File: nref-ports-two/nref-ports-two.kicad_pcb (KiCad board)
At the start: 4 copper layers, 87.5 x 40.2 mm, 117 parts, among them J1 USB_C_Receptacle, J2 USB_C_Receptacle, J3 USB3_A, J4 HD0919MSMTTR, J5 Conn_01x20, J6 Conn_01x12_Pin, J7 Conn_01x04, U1 TUSB8041, U10 TPD4E02B04DQA, U11 TPD12S521, U12 LM2830XQMFE/NOPB, U13 LM2830XQMFE/NOPB, U2 HD3SS3220IRNHT, U3 TPD4E02B04DQA, U4 TPD4E02B04DQA, U5 TPD4E02B04DQA, U6 TPD4E02B04DQA, U7 TPD4E02B04DQA, U8 TPD4E02B04DQA, U9 TPD4E02B04DQA, Y1 24MHz

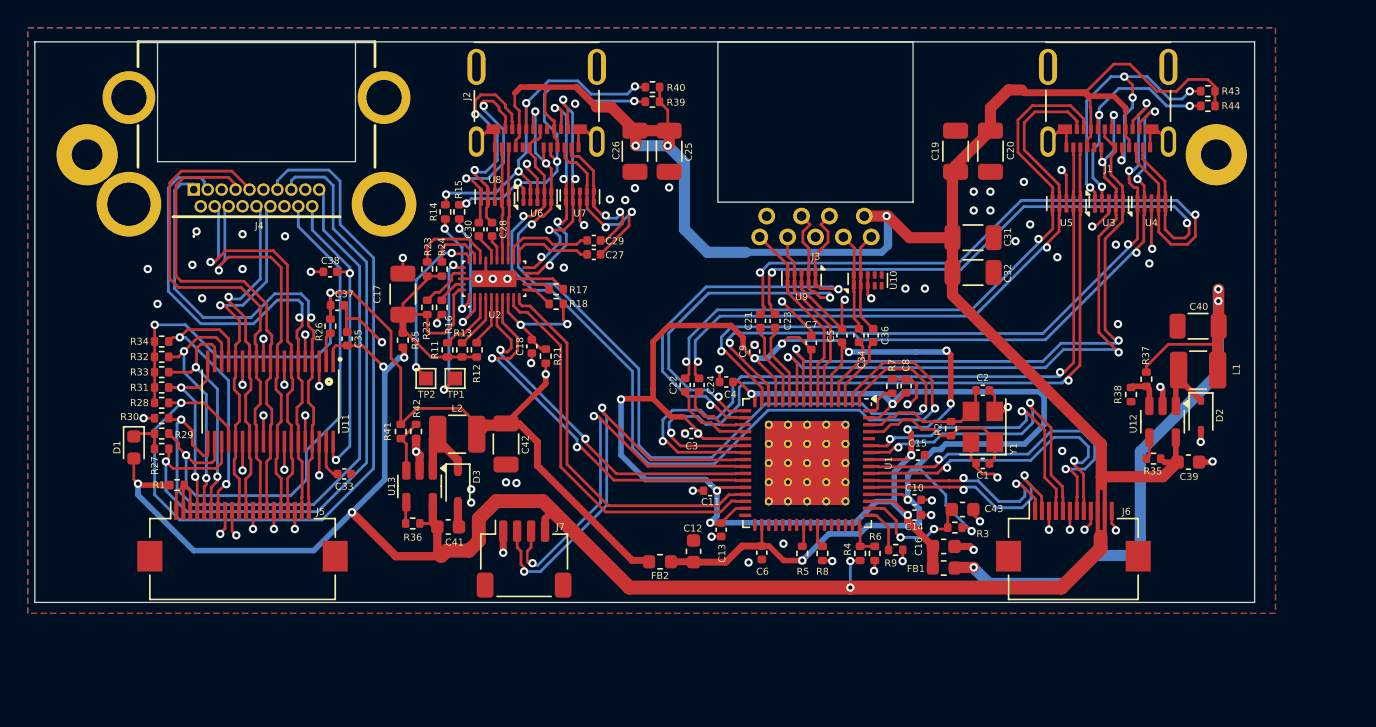
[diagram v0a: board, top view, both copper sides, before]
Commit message: WIP ports-two redesign
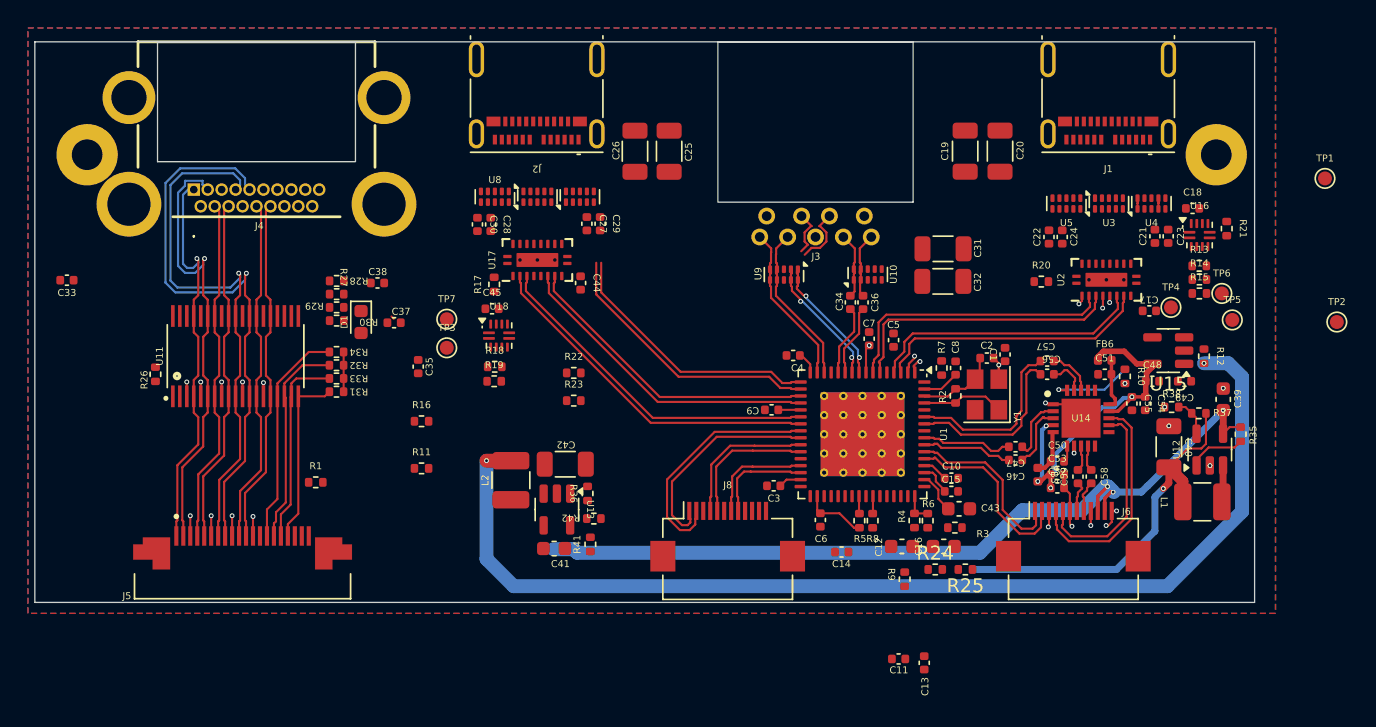
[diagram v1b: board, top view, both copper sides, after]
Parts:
- removed D2, D3: PMEG1020EA,115, Diode_SMD:D_SOD-323
- removed FB1, FB2: 220@100MHz 1.4A, Inductor_SMD:L_0603_1608Metric
- removed J7: Conn_01x04, Connector_JST:JST_SH_SM04B-SRSS-TB_1x04-1MP_P1.00mm_Horizontal
- removed R39, R40, R43, R44: 22k, Resistor_SMD:R_0402_1005Metric
- added C44: 0.1uF, Capacitor_SMD:C_0402_1005Metric, F.Cu at (139.2, 97.3)
- added C45: 0.1uF, Capacitor_SMD:C_0402_1005Metric, F.Cu at (132.8, 99.2)
- added C46: 0.1uF, Capacitor_SMD:C_0402_1005Metric, F.Cu at (170.3, 110.0)
- added C47: 0.1uF, Capacitor_SMD:C_0402_1005Metric, F.Cu at (170.3, 109.0)
- added C48: 1uF, Capacitor_SMD:C_0402_1005Metric, F.Cu at (180.2, 104.3)
- added C49: 1uF, Capacitor_SMD:C_0402_1005Metric, F.Cu at (182.5, 104.3)
- added C50: 4.7uF, Capacitor_SMD:C_0402_1005Metric, F.Cu at (173.3, 110.1)
- added C51: 4.7uF, Capacitor_SMD:C_0402_1005Metric, F.Cu at (176.8, 103.8)
- added C52: 0.1uF, Capacitor_SMD:C_0402_1005Metric, F.Cu at (173.3, 112.0)
- added C53: 1uF, Capacitor_SMD:C_0402_1005Metric, F.Cu at (173.3, 111.0)
- added C54: 1uF, Capacitor_SMD:C_0402_1005Metric, F.Cu at (179.7, 106.0)
- added C55: 0.1uF, Capacitor_SMD:C_0402_1005Metric, F.Cu at (178.7, 106.0)
- added C56: 0.1uF, Capacitor_SMD:C_0402_1005Metric, F.Cu at (172.6, 103.8)
- added C57: 0.1uF, Capacitor_SMD:C_0402_1005Metric, F.Cu at (172.6, 102.9)
- added C58: 0.1uF, Capacitor_SMD:C_0402_1005Metric, F.Cu at (175.8, 111.2)
- added C59: 0.1uF, Capacitor_SMD:C_0402_1005Metric, F.Cu at (174.8, 111.2)
- added FB5: 100@100MHz 3A, Inductor_SMD:L_0402_1005Metric, F.Cu at (171.9, 111.0)
- added FB6: 100@100MHz 3A, Inductor_SMD:L_0402_1005Metric, F.Cu at (176.8, 102.8)
- added J8: Conn_01x12_Pin, Connector_FFC-FPC:Hirose_FH12-12S-0.5SH_1x12-1MP_P0.50mm_Horizontal, F.Cu at (149.7, 115.5)
- added R10: 0, Resistor_SMD:R_0402_1005Metric, F.Cu at (178.2, 104.0)
- added R19: 900k, Resistor_SMD:R_0402_1005Metric, F.Cu at (132.9, 104.3)
- added R20: 0, Resistor_SMD:R_0402_1005Metric, F.Cu at (172.2, 97.2)
- added TP3: TestPoint, TestPoint:TestPoint_Pad_D1.0mm, F.Cu at (129.6, 102.0)
- added TP4: TestPoint, TestPoint:TestPoint_Pad_D1.0mm, F.Cu at (181.5, 99.0)
- added TP5: TestPoint, TestPoint:TestPoint_Pad_D1.0mm, F.Cu at (185.9, 100.0)
- added TP6: TestPoint, TestPoint:TestPoint_Pad_D1.0mm, F.Cu at (185.2, 98.0)
- added TP7: TestPoint, TestPoint:TestPoint_Pad_D1.0mm, F.Cu at (129.6, 99.9)
- added U14: EQCO5X31C0-I_6NX, footprints:QFN50P400X400X100-21N-D, F.Cu at (175.1, 107.0)
- added U15: LP5907MFX-1.2, Package_TO_SOT_SMD:SOT-23-5, F.Cu at (181.3, 102.2)
- added U16: TUSB321, Package_DFN_QFN:Texas_X2QFN-12_1.6x1.6mm_P0.4mm, F.Cu at (183.6, 93.9)
- added U17: TMUXHS4212, footprints:Texas-VQFN20_2.5x4.5mm_RKS, F.Cu at (136.1, 95.7)
- added U18: TUSB321, Package_DFN_QFN:Texas_X2QFN-12_1.6x1.6mm_P0.4mm, F.Cu at (133.3, 101.1)
- C17: value 47uF -> 0.1uF; footprint Capacitor_SMD:C_1206_3216Metric -> Capacitor_SMD:C_0402_1005Metric
- J1, J2: footprint footprints:MOLEX_105450-0101 -> Connector_USB:USB_C_Receptacle_Molex_105450-0101
- J5: footprint Connector_FFC-FPC:Hirose_FH12-20S-0.5SH_1x20-1MP_P0.50mm_Horizontal -> footprints:AMPHENOL_SFV20R-2STE1HLF
- R11: value 10k -> 0
- R12: value 900k -> 10k
- R13, R22: value 200k -> 10k
- R14: value 0 -> 4.7k
- R15: value 0 -> 900k
- R18, R24: value 200k -> 0
- R23: value 200k -> 4.7k
- R31, R35, R36: value 100k -> 10k
- TP1, TP2: footprint TestPoint:TestPoint_Pad_1.0x1.0mm -> TestPoint:TestPoint_Pad_D1.0mm
- U12, U13: value LM2830XQMFE/NOPB -> TLV62569DBV
- U2: value HD3SS3220IRNHT -> TMUXHS4212; footprint footprints:QFN40P450X250X80-31N120X320 -> footprints:Texas-VQFN20_2.5x4.5mm_RKS
- moved TP2 65.5 mm to (193.4, 100.1)
- moved TP1 64.0 mm to (192.6, 89.8)
- moved R14 54.3 mm to (183.5, 97.0), turned to 0 degrees
- moved C17 53.6 mm to (179.9, 99.3), turned to 0 degrees
- moved R15 53.4 mm to (183.5, 98.0), turned to 0 degrees
- moved R13 53.2 mm to (183.5, 96.1), turned to 0 degrees
- moved R12 52.2 mm to (183.9, 102.5), turned to -90 degrees
- moved R21 49.7 mm to (185.5, 93.4)
- moved C18 48.4 mm to (183.1, 92.0), turned to 0 degrees
- moved U2 43.9 mm to (176.9, 97.1)
- moved R25 43.6 mm to (166.8, 117.8), turned to 180 degrees
- moved R24 41.4 mm to (164.6, 117.8), turned to 0 degrees
- moved C21 28.9 mm to (180.3, 94.0)
- moved C23 28.8 mm to (181.3, 94.0)
- moved C22 28.2 mm to (172.8, 94.0)
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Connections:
- net /USB3_1_SSTXCN renamed /USBH3_TXCN
- net /USB3_1_SSTXCP renamed /USBH3_TXCP
- net /USBH_1A_AC_TXN renamed /USBC2A_TXCN
- net /USBH_1A_AC_TXP renamed /USBC2A_TXCP
- net /USBH_1B_AC_TXN renamed /USBC2B_TXCN
- net /USBH_1B_AC_TXP renamed /USBC2B_TXCP
- net /USBH_2A_AC_TXN renamed /USBC1A_TXCN
- net /USBH_2A_AC_TXP renamed /USBC1A_TXCP
- net /USBH_2B_AC_TXN renamed /USBC1B_TXCN
- net /USBH_2B_AC_TXP renamed /USBC1B_TXCP
- net CC1 renamed USBC1_CC1
- net CC2 renamed USBC1_CC2
- C17 pad 1: MUX_5V -> /MUX_3V3
- C18 pad 1: MUX_3V3 -> +5V
- C21 pad 2: USBH_2A_TXN -> USBC1A_TXN
- C22 pad 2: USBH_2B_TXN -> USBC1B_TXN
- C23 pad 2: USBH_2A_TXP -> USBC1A_TXP
- C24 pad 2: USBH_2B_TXP -> USBC1B_TXP
- C27 pad 2: USBH_MUXA_TXN -> USBC2A_TXN
- C28 pad 2: USBH_MUXB_TXN -> USBC2B_TXN
- C29 pad 2: USBH_MUXA_TXP -> USBC2A_TXP
- C30 pad 2: USBH_MUXB_TXP -> USBC2B_TXP
- C34 pad 1: USBH_1A_TXN -> USBH3_TXN
- C36 pad 1: USBH_1A_TXP -> USBH3_TXP
- J1 pad A10: USBH_2B_RXN -> USBC1B_RXN
- J1 pad A11: USBH_2B_RXP -> USBC1B_RXP
- J1 pad A6: USBH_2_DP -> USBC1_DP
- J1 pad A7: USBH_2_DN -> USBC1_DN
- J1 pad B10: USBH_2A_RXN -> USBC1A_RXN
- J1 pad B11: USBH_2A_RXP -> USBC1A_RXP
- J1 pad B6: USBH_2_DP -> USBC1_DP
- J1 pad B7: USBH_2_DN -> USBC1_DN
- J2 pad A10: USBH_MUXB_RXN -> USBC2B_RXN
- J2 pad A11: USBH_MUXB_RXP -> USBC2B_RXP
- J2 pad A5: MUXCC1 -> USBC2_CC1
- J2 pad A6: USBH_1_DP -> USBC2_DP
- J2 pad A7: USBH_1_DN -> USBC2_DN
- J2 pad B10: USBH_MUXA_RXN -> USBC2A_RXN
- J2 pad B11: USBH_MUXA_RXP -> USBC2A_RXP
- J2 pad B5: MUXCC2 -> USBC2_CC2
- J2 pad B6: USBH_1_DP -> USBC2_DP
- J2 pad B7: USBH_1_DN -> USBC2_DN
- J3 pad 5: USBH_1A_RXN -> USBH3_RXN
- J3 pad 6: USBH_1A_RXP -> USBH3_RXP
- J5 pad 1: Net-(J5-Pin_1) -> HDMI_TX2P
- J5 pad 10: HDMI_CLKN -> HDMI_CLKP
- J5 pad 11: HDMI_CLKP -> HDMI_CLKN
- J5 pad 13: HDMI_TX0N -> GND
- J5 pad 14: HDMI_TX0P -> HDMI_CEC
- J5 pad 15: GND -> HDMI_SCL
- J5 pad 16: HDMI_TX1N -> HDMI_SDA
- J5 pad 17: HDMI_TX1P -> HDMI_HPD
- J5 pad 18: GND -> Net-(J5-Pin_18)
- J5 pad 19: HDMI_TX2N -> Net-(J5-Pin_18)
- J5 pad 2: Net-(J5-Pin_1) -> HDMI_TX2N
- J5 pad 20: HDMI_TX2P -> Net-(J5-Pin_18)
- J5 pad 3: Net-(J5-Pin_1) -> GND
- J5 pad 4: HDMI_HPD -> HDMI_TX1P
- J5 pad 5: HDMI_SCL -> HDMI_TX1N
- J5 pad 6: HDMI_SDA -> GND
- J5 pad 7: HDMI_CEC -> HDMI_TX0P
- J5 pad 8: GND -> HDMI_TX0N
- L1 pad 1: Net-(D2-K) -> Net-(U12-SW)
- L2 pad 1: Net-(D3-K) -> Net-(U13-SW)
- R1 pad 1: Net-(J5-Pin_1) -> Net-(J5-Pin_18)
- R11 pad 1: MUX_5V -> /MUX_3V3
- R11 pad 2: Net-(U2-CURRENT_MODE) -> +3V3
- R12 pad 1: MUX_5V -> Net-(U15-EN)
- R12 pad 2: Net-(U2-VBUS_DET) -> +3V3
- R13 pad 1: MUX_5V -> +5V
- R13 pad 2: Net-(U2-PORT) -> Net-(U16-CURRENT_MODE)
- R14 pad 1: MUXCC2 -> +5V
- R14 pad 2: Net-(U2-CC2) -> Net-(U16-PORT)
- R15 pad 1: MUXCC1 -> +5V
- R15 pad 2: Net-(U2-CC1) -> Net-(U16-VBUS_DET)
- R16 pad 1: GND -> /MUX_3V3
- R16 pad 2: Net-(U2-~{ENN_CC}) -> +3V3
- R17 pad 1: GND -> ~{USB_MUX_OE}
- R17 pad 2: Net-(U2-~{ENN_MUX}) -> Net-(U17-~{OE})
- R18 pad 1: Net-(U2-DIR) -> USBC2_MUX_DIR
- R18 pad 2: MUX_3V3 -> Net-(U17-SEL)
- R21 pad 1: MUX_3V3 -> USBC1_MUX_DIR
- R21 pad 2: +3V3 -> Net-(U2-SEL)
- R22 pad 1: Net-(U2-ID) -> +5V
- R22 pad 2: MUX_5V -> Net-(U18-CURRENT_MODE)
- R23 pad 1: Net-(U2-~{INT_N}/OUT3) -> +5V
- R23 pad 2: MUX_5V -> Net-(U18-PORT)
- R24 pad 1: Net-(U2-VCONN_FAULT_N) -> +3V3
- R24 pad 2: MUX_5V -> USBH_3V3
- R25 pad 1: MUX_5V -> +1V1
- R25 pad 2: +5V -> USBH_1V1
- TP1 pad 1: Net-(U2-SCL/OUT2) -> Net-(U16-ID)
- TP2 pad 1: Net-(U2-SDA/OUT1) -> Net-(U16-~{VCONN_FAULT})
- U1 pad 1: USBH_1_DP -> USBC1_DP
- U1 pad 10: USBH_2_DN -> USBH_3_DN
- U1 pad 11: USBH_2A_TXP -> USBH3_TXP
- U1 pad 12: USBH_2A_TXN -> USBH3_TXN
- U1 pad 14: USBH_2A_RXP -> USBH3_RXP
- U1 pad 15: USBH_2A_RXN -> USBH3_RXN
- U1 pad 17: USBH_3_DP -> USBC2_DP
- U1 pad 18: USBH_3_DN -> USBC2_DN
- U1 pad 19: USBH_2B_TXP -> USBH2_TXP
- U1 pad 2: USBH_1_DN -> USBC1_DN
- U1 pad 20: USBH_2B_TXN -> USBH2_TXN
- U1 pad 22: USBH_2B_RXN -> USBH2_RXP
- U1 pad 23: USBH_2B_RXP -> USBH2_RXN
- U1 pad 26: USBH_1B_TXP -> USBH4_TXN
- U1 pad 27: USBH_1B_TXN -> USBH4_TXP
- U1 pad 29: USBH_1B_RXN -> USBH4_RXN
- U1 pad 3: USBH_1A_TXP -> USBH1_TXP
- U1 pad 30: USBH_1B_RXP -> USBH4_RXP
- U1 pad 4: USBH_1A_TXN -> USBH1_TXN
- U1 pad 55: USB2_RXP -> /UP_SSTXP
- U1 pad 56: USB2_RXN -> /UP_SSTXN
- U1 pad 58: USB2_TXP -> USB2_RE_TXN
- U1 pad 59: USB2_TXN -> USB2_RE_TXP
- U1 pad 6: USBH_1A_RXP -> USBH1_RXP
- U1 pad 7: USBH_1A_RXN -> USBH1_RXN
- U1 pad 9: USBH_2_DP -> USBH_3_DP
- U12 pad 1: Net-(D2-K) -> Net-(U12-EN)
- U12 pad 3: Net-(U12-FB) -> Net-(U12-SW)
- U12 pad 4: Net-(U12-EN) -> +5V
- U12 pad 5: +5V -> Net-(U12-FB)
- U13 pad 1: Net-(D3-K) -> Net-(U13-EN)
- U13 pad 3: Net-(U13-FB) -> Net-(U13-SW)
- U13 pad 4: Net-(U13-EN) -> +5V
- U13 pad 5: +5V -> Net-(U13-FB)
- U2 pad 1: Net-(U2-CC2) -> unconnected-(U2-RSVD1-Pad1)
- U2 pad 10: USBH_1B_RXN -> unconnected-(U2-RSVD2-Pad10)
- U2 pad 11: Net-(U2-DIR) -> GND
- U2 pad 12: Net-(U2-~{ENN_MUX}) -> USBC1B_TXP
- U2 pad 13: GND -> USBC1B_TXN
- U2 pad 14: USBH_MUXA_RXN -> USBC1B_RXP
- U2 pad 15: USBH_MUXA_RXP -> USBC1B_RXN
- U2 pad 16: USBH_MUXA_TXN -> USBC1A_TXN
- U2 pad 17: USBH_MUXA_TXP -> USBC1A_TXP
- U2 pad 18: USBH_MUXB_RXN -> USBC1A_RXN
- U2 pad 19: USBH_MUXB_RXP -> USBC1A_RXP
- U2 pad 2: Net-(U2-CC1) -> Net-(U2-~{OE})
- U2 pad 20: USBH_MUXB_TXN -> GND
- U2 pad 3: Net-(U2-CURRENT_MODE) -> USBH1_RXN
- U2 pad 4: Net-(U2-PORT) -> USBH1_RXP
- U2 pad 5: Net-(U2-VBUS_DET) -> GND
- U2 pad 6: USBH_1B_TXP -> /MUX_3V3
- U2 pad 7: USBH_1B_TXN -> USBH1_TXN
- U2 pad 8: MUX_3V3 -> USBH1_TXP
- U2 pad 9: USBH_1B_RXP -> Net-(U2-SEL)
- U3 pad 4: USBH_2_DN -> USBC1_DN
- U3 pad 5: USBH_2_DP -> USBC1_DP
- U3 pad 6: USBH_2_DP -> USBC1_DP
- U3 pad 7: USBH_2_DN -> USBC1_DN
- U4 pad 1: USBH_2A_RXN -> USBC1A_RXN
- U4 pad 10: USBH_2A_RXN -> USBC1A_RXN
- U4 pad 2: USBH_2A_RXP -> USBC1A_RXP
- U4 pad 9: USBH_2A_RXP -> USBC1A_RXP
- U5 pad 1: USBH_2B_RXN -> USBC1B_RXN
- U5 pad 10: USBH_2B_RXN -> USBC1B_RXN
- U5 pad 2: USBH_2B_RXP -> USBC1B_RXP
- U5 pad 9: USBH_2B_RXP -> USBC1B_RXP
- U6 pad 1: MUXCC1 -> USBC2_CC1
- U6 pad 10: MUXCC1 -> USBC2_CC1
- U6 pad 2: MUXCC2 -> USBC2_CC2
- U6 pad 4: USBH_1_DN -> USBC2_DN
- U6 pad 5: USBH_1_DP -> USBC2_DP
- U6 pad 6: USBH_1_DP -> USBC2_DP
- U6 pad 7: USBH_1_DN -> USBC2_DN
- U6 pad 9: MUXCC2 -> USBC2_CC2
- U7 pad 1: USBH_MUXA_RXN -> USBC2A_RXN
- U7 pad 10: USBH_MUXA_RXN -> USBC2A_RXN
- U7 pad 2: USBH_MUXA_RXP -> USBC2A_RXP
- U7 pad 9: USBH_MUXA_RXP -> USBC2A_RXP
- U8 pad 1: USBH_MUXB_RXN -> USBC2B_RXN
- U8 pad 10: USBH_MUXB_RXN -> USBC2B_RXN
- U8 pad 2: USBH_MUXB_RXP -> USBC2B_RXP
- U8 pad 9: USBH_MUXB_RXP -> USBC2B_RXP
- U9 pad 1: USBH_3_DN -> USBH_3_DP
- U9 pad 10: USBH_3_DN -> USBH_3_DP
- U9 pad 2: USBH_3_DP -> USBH_3_DN
- U9 pad 4: USBH_1A_RXP -> USBH3_RXP
- U9 pad 5: USBH_1A_RXN -> USBH3_RXN
- U9 pad 6: USBH_1A_RXN -> USBH3_RXN
- U9 pad 7: USBH_1A_RXP -> USBH3_RXP
- U9 pad 9: USBH_3_DP -> USBH_3_DN
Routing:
- net +5V: track 256.6 -> 60.2 mm, vias 9 -> 3
- net USBH_1V1: track 113.2 -> 7.58 mm, vias 12 -> 1
- net GND: track 122.1 -> 25.6 mm, vias 90 -> 22
- net USBH_3V3: track 77.4 -> 10.6 mm, vias 5 -> 0
- net USBH_1_DP: track 63.9 -> 0.00 mm, vias 4 -> 0
- net USBH_1_DN: track 63.8 -> 0.00 mm, vias 2 -> 0
- net Net-(J4-CEC): track 58.8 -> 0.00 mm, vias 1 -> 0
- net USBH_2B_RXP: track 55.8 -> 0.00 mm, vias 2 -> 0
- net USBH_2B_RXN: track 54.9 -> 0.00 mm, vias 2 -> 0
- net USBH_2A_RXN: track 52.5 -> 0.00 mm, vias 4 -> 0
- net USBH_2A_RXP: track 51.2 -> 0.00 mm, vias 4 -> 0
- net Net-(J4-SCL): track 50.3 -> 0.00 mm, vias 1 -> 0
- net USBH_2_DN: track 49.4 -> 0.00 mm, vias 4 -> 0
- net /USBC1A_TXCN: track 48.6 -> 0.79 mm, vias 2 -> 0
- net /USBC1B_TXCN: track 47.8 -> 0.00 mm, vias 2 -> 0
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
